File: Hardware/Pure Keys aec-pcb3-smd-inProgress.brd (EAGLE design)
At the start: 162.5 x 51.7 mm, 72 parts, among them Q2 20MHz, U1 ATMEGA328P_TQFP

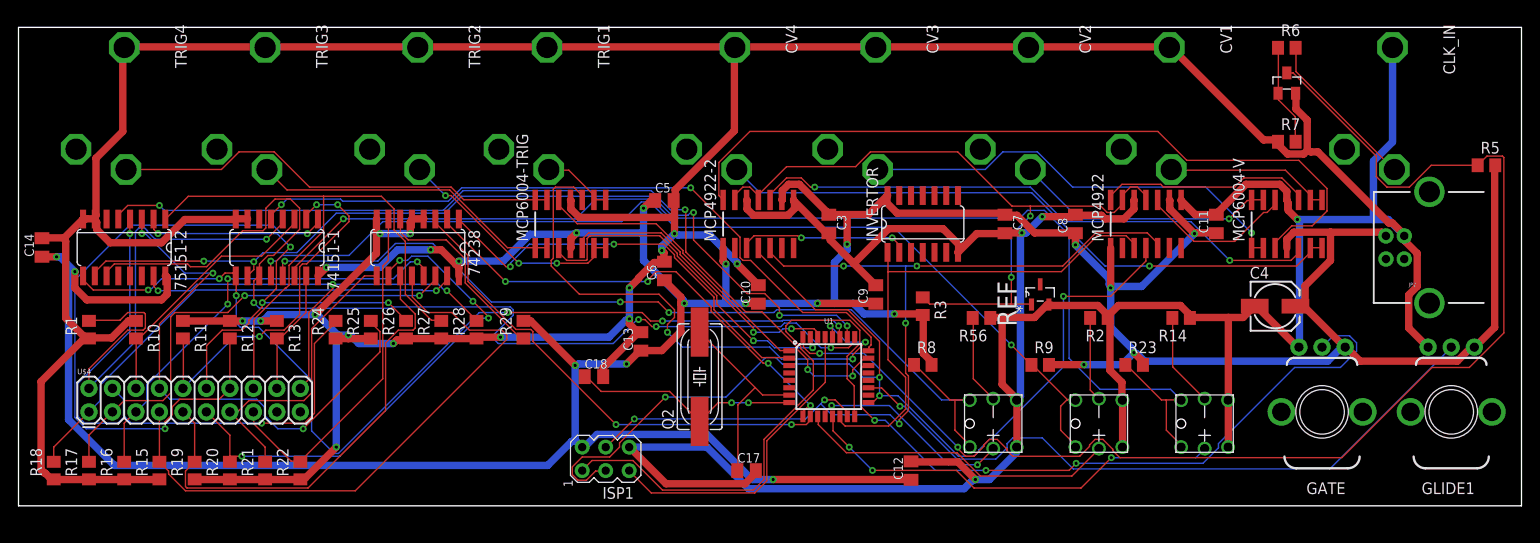
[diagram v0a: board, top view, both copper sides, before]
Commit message: reroutes
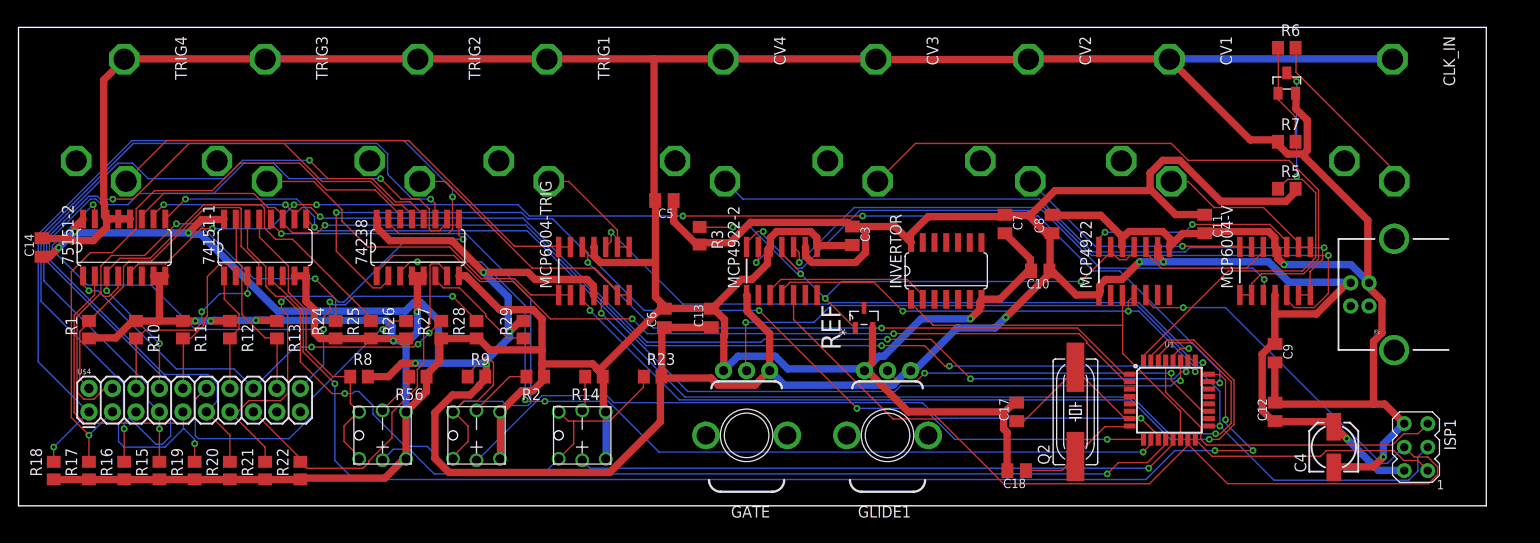
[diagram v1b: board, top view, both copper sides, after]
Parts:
- moved ISP1 87.6 mm to (151.1, 0.00), turned to 180 degrees
- moved BUT2 67.3 mm to (49.5, 1.27)
- moved BUT3 67.3 mm to (61.0, 1.27)
- moved BUT1 66.1 mm to (39.4, 1.27)
- moved R14 63.8 mm to (62.2, 7.62)
- moved GATE 62.3 mm to (78.7, 1.27)
- moved R2 61.3 mm to (55.9, 7.62)
- moved R56 61.3 mm to (43.2, 7.62)
- moved GLIDE1 61.0 mm to (94.0, 1.27)
- moved R8 61.0 mm to (36.8, 7.62)
- moved R9 61.0 mm to (49.5, 7.62)
- moved R23 52.1 mm to (68.6, 7.62)
- moved C18 46.8 mm to (108.0, -2.54), turned to 180 degrees
- moved C9 43.6 mm to (135.9, 10.2), turned to 270 degrees
- moved Q2 40.8 mm to (114.3, 3.81)
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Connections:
- net 5V: now also U1.6
- net GND: now also 75151-2.12, 75151-2.13, 75151-2.14, U1.21
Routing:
- net CLK_IN: track 141.2 -> 47.7 mm
- net GND: track 725.4 -> 642.3 mm, vias 18 -> 8
- net BUTLED1: track 22.3 -> 88.1 mm, vias 2 -> 1
- net BUT1: track 97.2 -> 32.9 mm, vias 3 -> 0
- net BUT3: track 130.8 -> 69.4 mm
- net A1OUT: track 50.8 -> 109.8 mm
- net TRIG2: track 32.4 -> 91.4 mm
- net DAIN: track 76.3 -> 135.2 mm, vias 2 -> 4
- net TRIG3: track 37.7 -> 94.9 mm
- net MK3: track 70.3 -> 13.3 mm, vias 2 -> 0
- net A2OUT: track 52.9 -> 97.4 mm, vias 2 -> 4
- net BUTLED2: track 34.8 -> 78.9 mm, vias 0 -> 1
- net A0OUT: track 45.2 -> 88.4 mm
- net T4: track 51.7 -> 92.7 mm, vias 0 -> 2
- net 5V: track 455.4 -> 414.7 mm, vias 21 -> 11
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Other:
- board size 162.5 x 51.7 mm -> 158.7 x 51.7 mm
